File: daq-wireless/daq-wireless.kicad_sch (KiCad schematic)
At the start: 30 parts, among them J1 5223004-2, J2 Micro_SD_Card, J3 USB_C_Receptacle_USB2.0, Q1 MMBT3904, Q2 MMBT3904, U1 ESP32-WROOM-32, U2 AMS1117, U3 FT231XS, U5 Ebyte_E01-ML01SP4

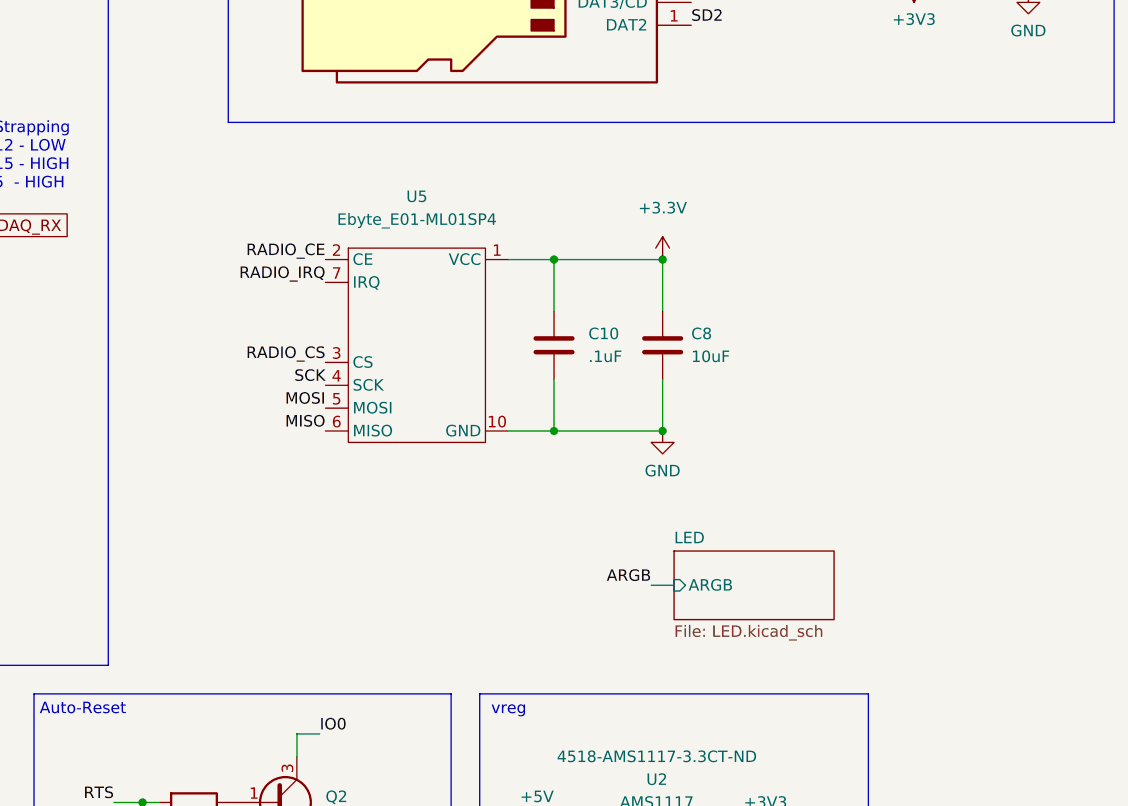
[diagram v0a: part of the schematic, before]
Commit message: DAQ updates
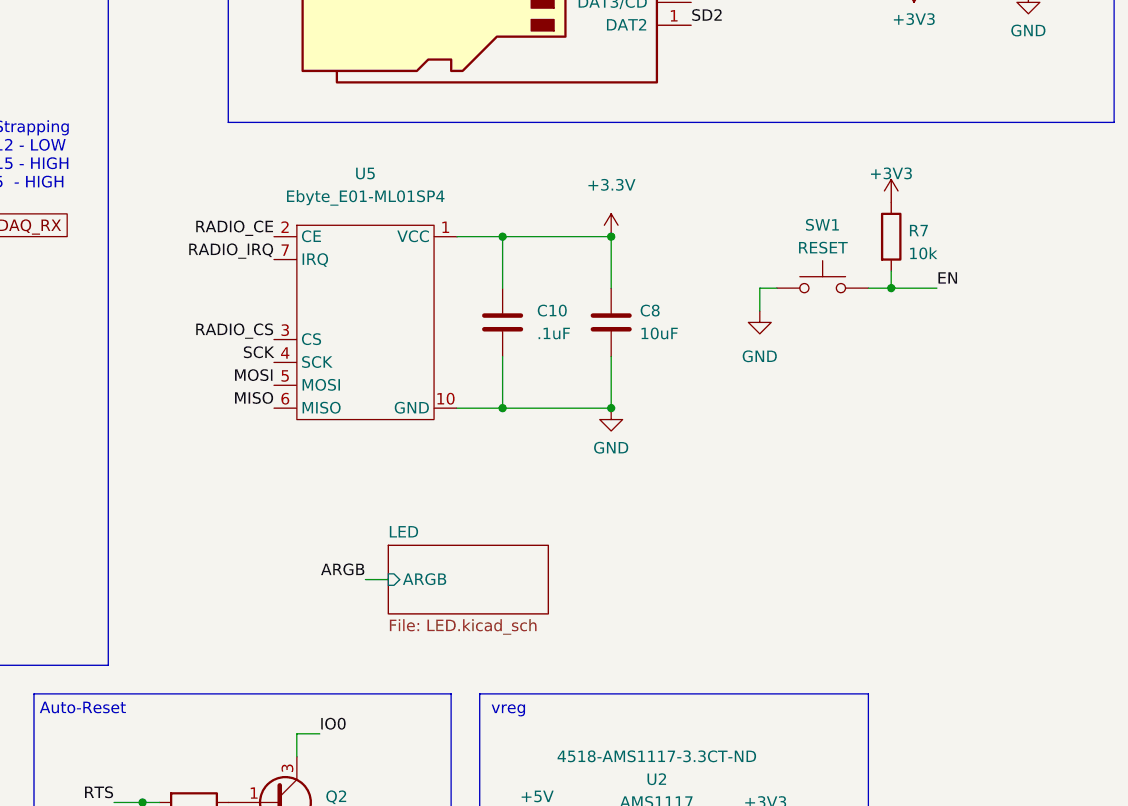
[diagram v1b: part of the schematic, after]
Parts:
- added R7: 10k, Resistor_SMD:R_0603_1608Metric, symbol Device:R
- added SW1: RESET, Button_Switch_THT:SW_PUSH_6mm, symbol Switch:SW_Push
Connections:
- net +3V3: now also R7.1
- net EN: now also R7.2, SW1.2
- net GND: now also SW1.1
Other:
- moved on the sheet: C10, C8, U5
